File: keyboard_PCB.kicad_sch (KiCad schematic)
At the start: 29 parts, among them J1 USB TYPE-C-31-M-12, J2 009159010061916, SW1 SW_Push, SW2 SW_Push, U1 USBLC6-2SC6, U2 TLV75733PDBV, U3 TLV75733PDBV, U4 STM32F446RETx, Y1 X322516MLB4SI

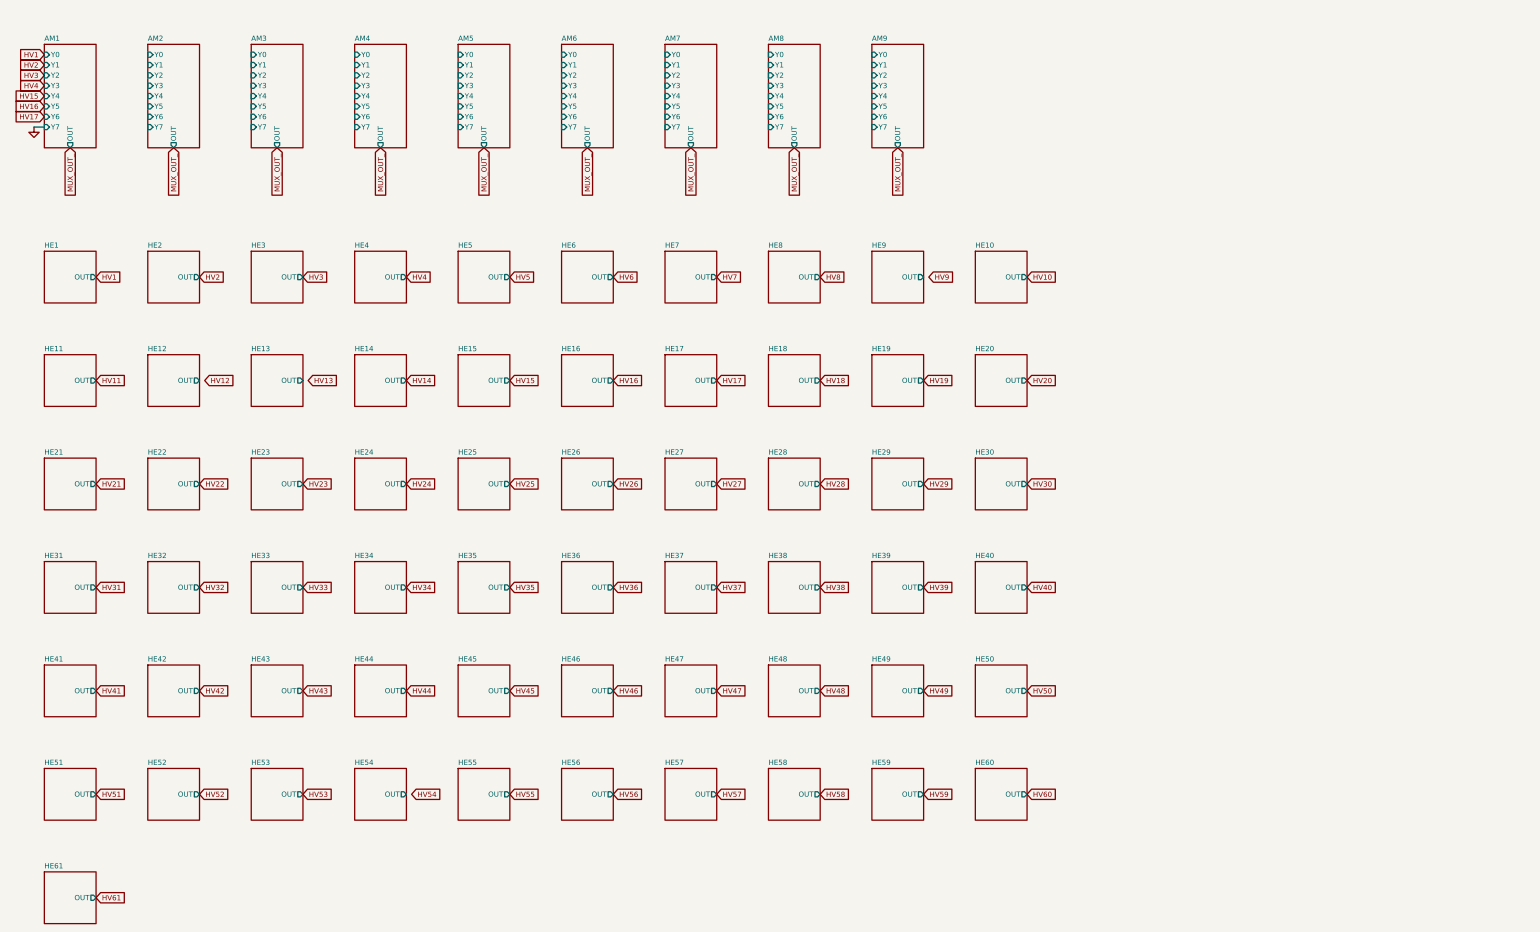
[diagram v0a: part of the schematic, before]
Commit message: sch done
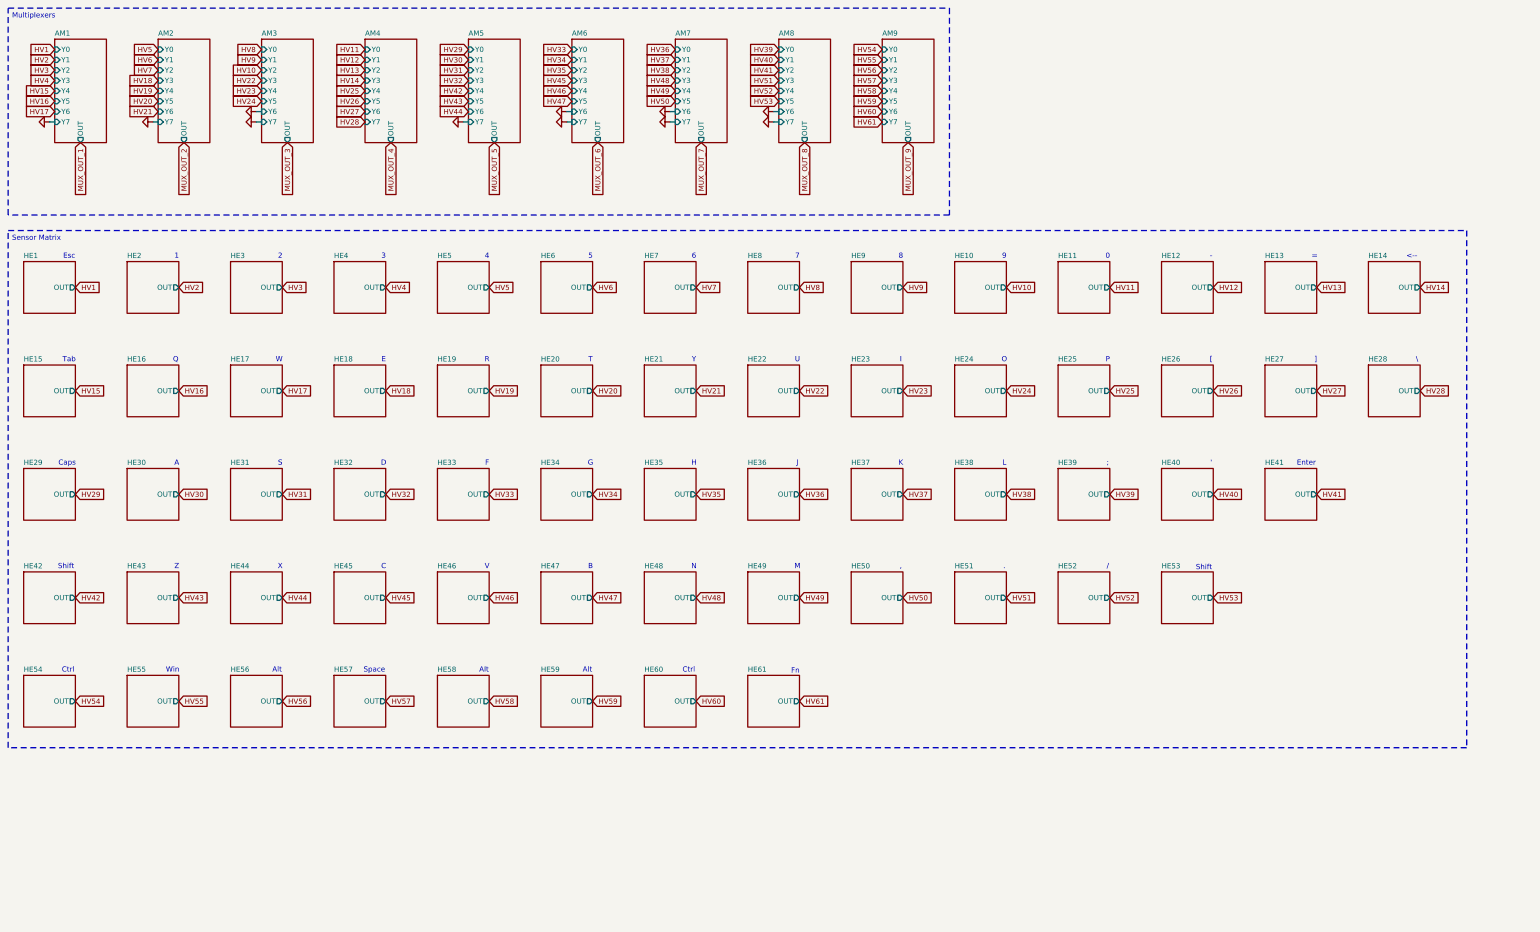
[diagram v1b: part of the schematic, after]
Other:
- note added: "'"
- note added: ","
- note added: "-"
- note added: "."
- note added: "/"
- note added: "0"
- note added: "1"
- note added: "2"
- note added: "3"
- note added: "4"
- note added: "5"
- note added: "6"
- note added: "7"
- note added: "8"
- note added: "9"
- note added: ";"
- note added: "<--"
- note added: "="
- note added: "A"
- note added: "Alt"
- note added: "B"
- note added: "C"
- note added: "Caps"
- note added: "Ctrl"
- note added: "D"
- note added: "E"
- note added: "Enter"
- note added: "Esc"
- note added: "F"
- note added: "Fn"
- note added: "G"
- note added: "H"
- note added: "I"
- note added: "J"
- note added: "K"
- note added: "L"
- note added: "M"
- note added: "N"
- note added: "O"
- note added: "P"
- note added: "Q"
- note added: "R"
- note added: "S"
- note added: "Shift"
- note added: "Space"
- note added: "T"
- note added: "Tab"
- note added: "U"
- note added: "V"
- note added: "W"
- note added: "Win"
- note added: "X"
- note added: "Y"
- note added: "Z"
- note added: "["
- note added: "\"
- note added: "]"
